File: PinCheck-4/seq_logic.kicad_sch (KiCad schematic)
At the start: 10 parts, among them J3 LEMHAL Header, U5 74HC14, U6 74HC14, U7 USBLC6-4SC6

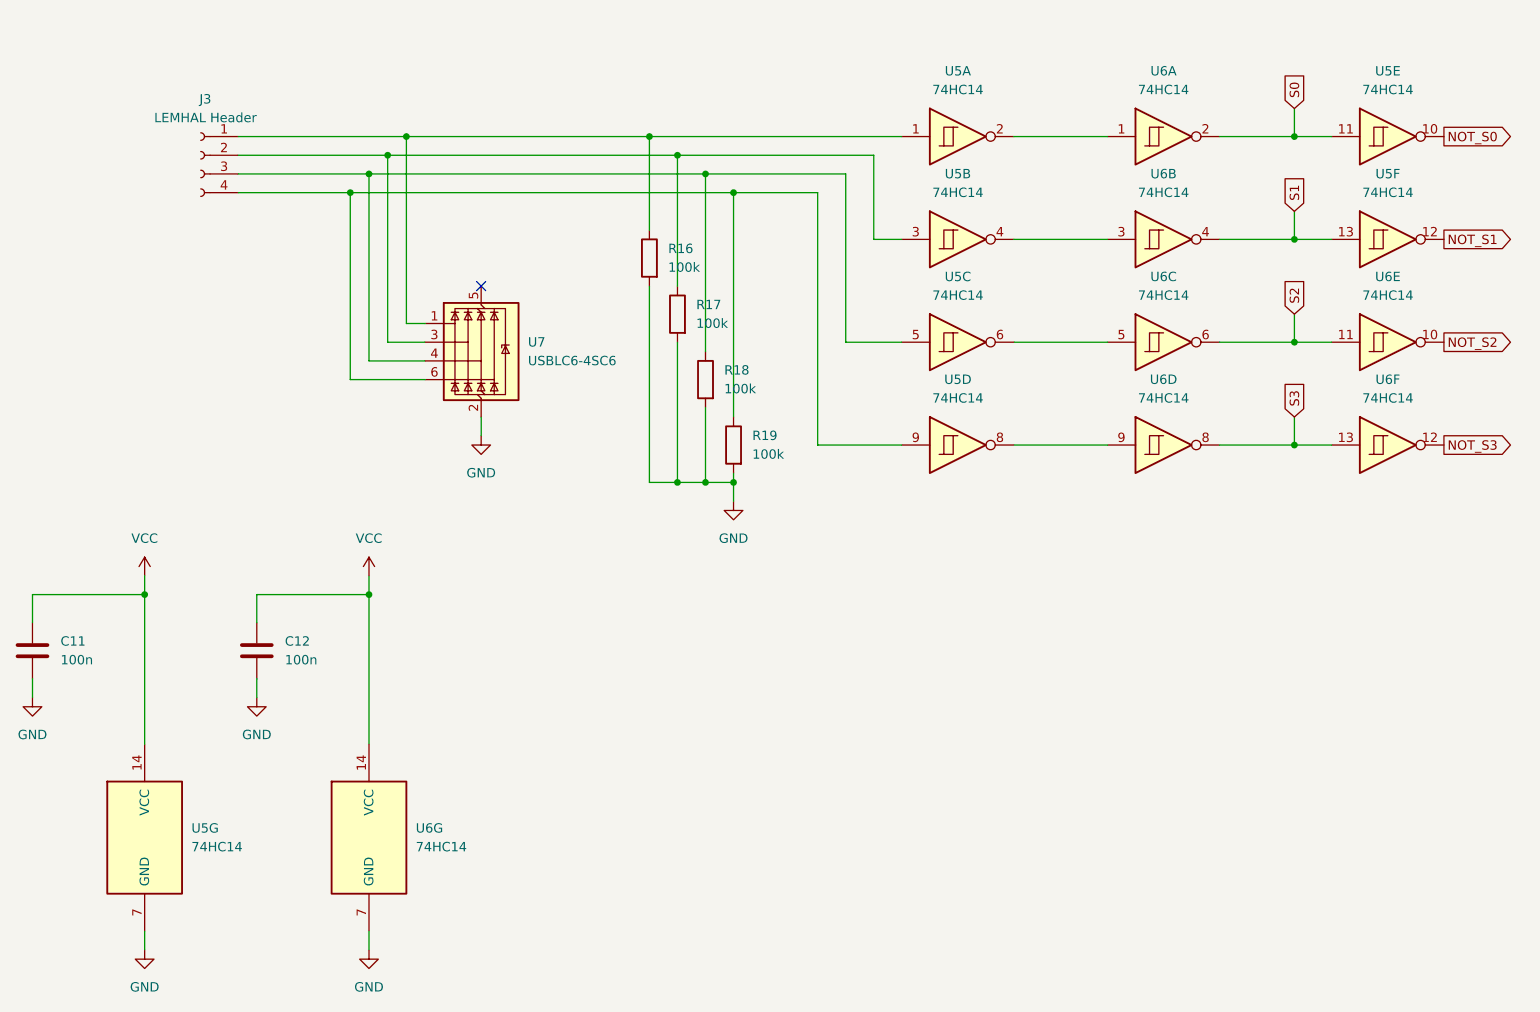
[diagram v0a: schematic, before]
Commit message: Daily sync 2025-08-28 16:55
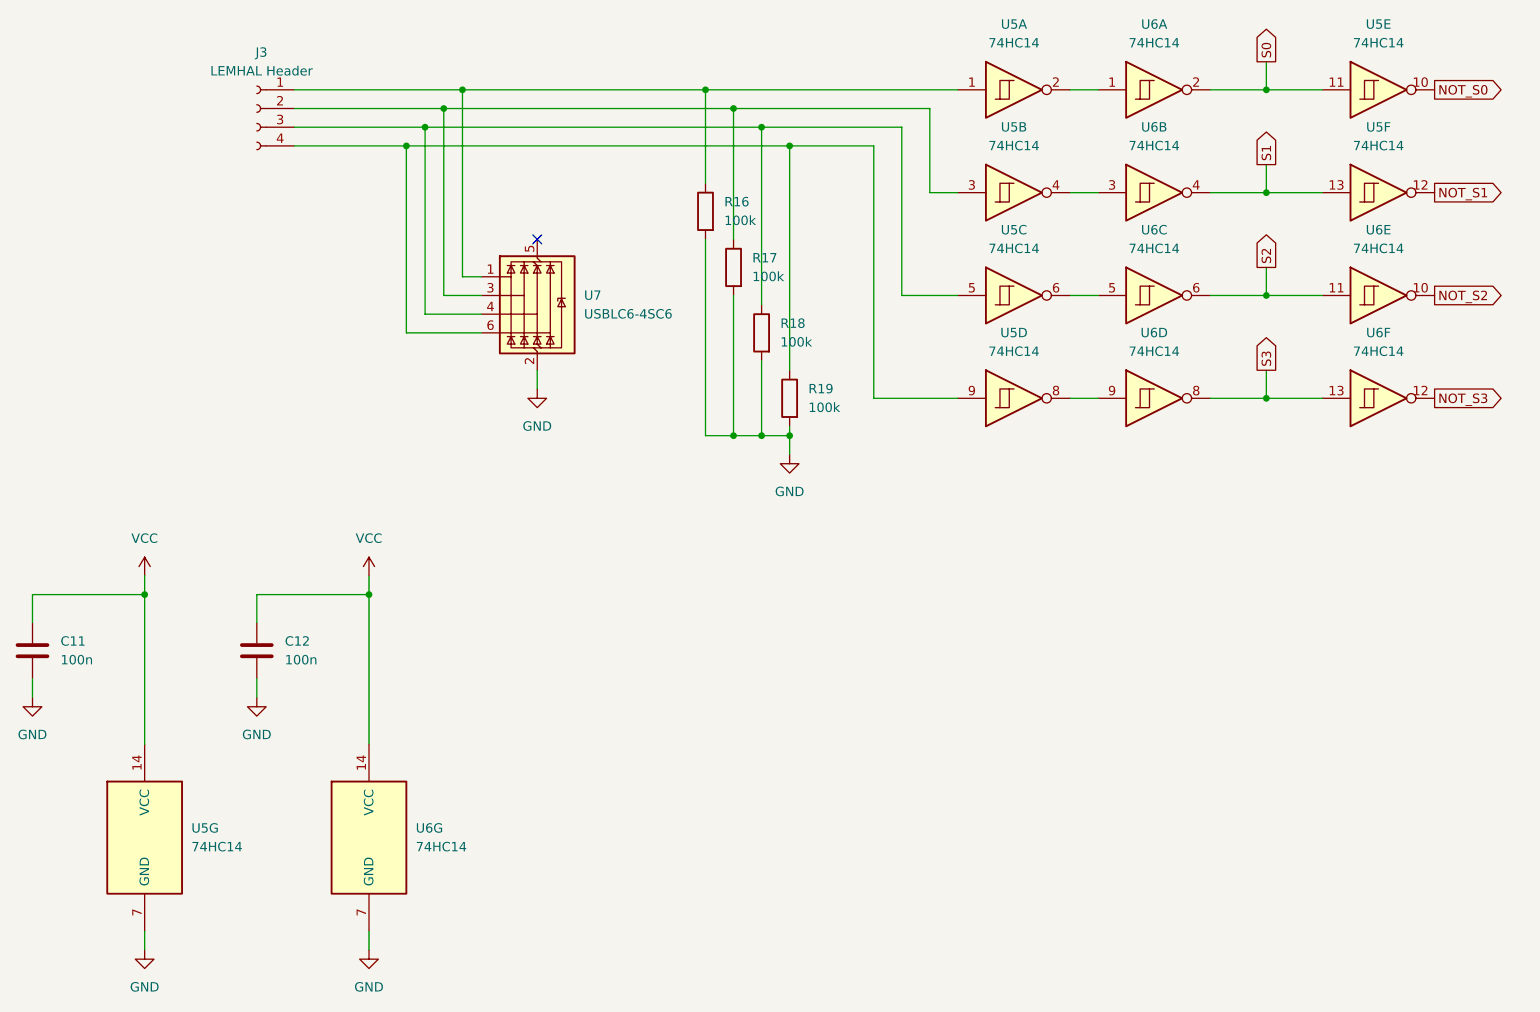
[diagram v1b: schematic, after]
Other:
- moved on the sheet: J3, R16, R17, R18, R19, U5A, U5B, U5C, U5D, U5E, U5F, U6A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

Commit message: Daily sync 2025-08-29 22:48
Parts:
- C11, C12: Manufacturer Part No (none) -> 0805B104K160CT
- J3: Manufacturer Part No (none) -> 26-60-5040
- R16, R17, R18, R19: Manufacturer Part No (none) -> ERJP6WF1003V
- U5, U6: Manufacturer Part No (none) -> 74HC14D
- U7: Manufacturer Part No (none) -> USBLC6-4SC6
